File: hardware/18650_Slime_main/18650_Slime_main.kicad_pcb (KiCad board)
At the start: 2 copper layers, 59.8 x 17 mm, 56 parts, among them J1 RJ12, J2 USB_C_Receptacle_USB2.0, J3 Conn_01x04_Male, Q1 2N3904, Q2 CJ2305, Q3 2N3904, Q4 CJ2305, SW1 SW_Push, SW2 SW_Push, SW3 SW_Push, U1 BMI160_Module, U2 ESP32-C3-MINI-1, U3 M3406, U4 SRV05-4, Y1 DNP

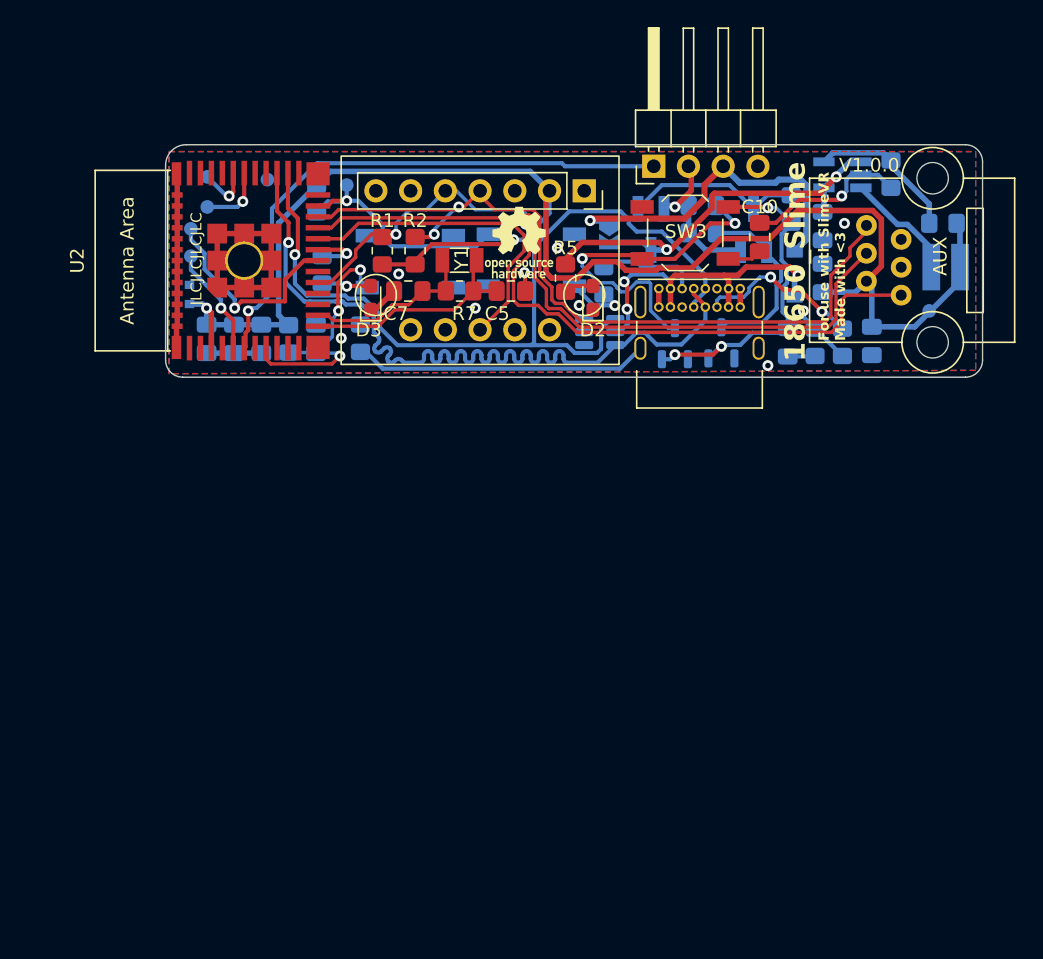
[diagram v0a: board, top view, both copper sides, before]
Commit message: V1.0.0 Release, UNTESTED
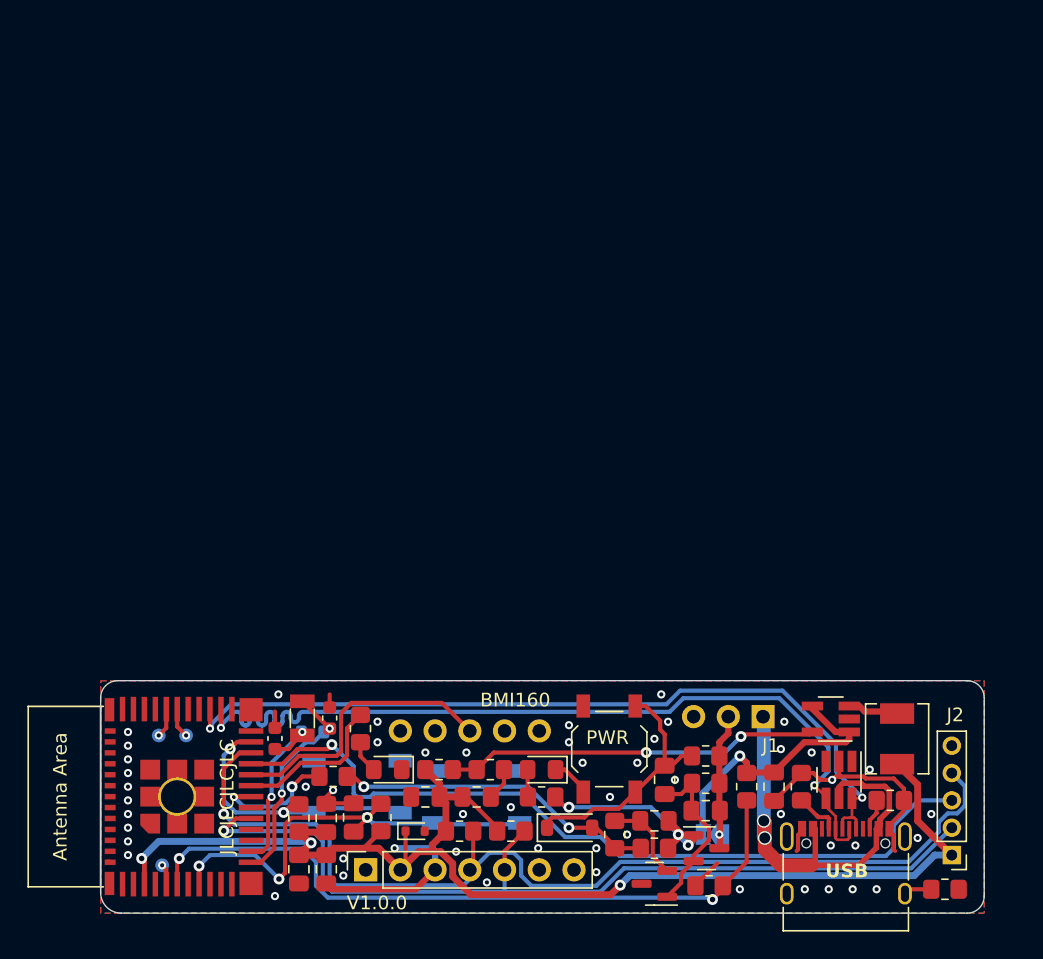
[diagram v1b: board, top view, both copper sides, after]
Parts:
- removed D4: B5819W, Diode_SMD:D_SOD-123
- removed the G*** at (89.6, 62.2)
- removed Q2, Q4: CJ2305, Package_TO_SOT_SMD:SOT-23_Handsoldering
- removed TP3: IO9, TestPoint:TestPoint_Pad_D1.0mm
- removed TP5: IO2, TestPoint:TestPoint_Pad_D1.0mm
- removed TP6: GND, TestPoint:TestPoint_Pad_D1.0mm
- removed TP7: 3v3, TestPoint:TestPoint_Pad_D1.0mm
- added C12: 100nF, Capacitor_SMD:C_0805_2012Metric_Pad1.18x1.45mm_HandSolder, F.Cu at (103.2, 103.8)
- added D5: B5819W, Diode_SMD:D_SOD-123, F.Cu at (93.3, 105.0)
- added G***: LOGO, 18650_Slime:OpenSourceLogo, B.Cu at (69.2, 102.5)
- added R17: 1K, Resistor_SMD:R_0805_2012Metric_Pad1.20x1.40mm_HandSolder, F.Cu at (76.0, 101.2)
- added R18: 120K, Resistor_SMD:R_0805_2012Metric_Pad1.20x1.40mm_HandSolder, F.Cu at (106.2, 102.0)
- added R19: 27K, Resistor_SMD:R_0805_2012Metric_Pad1.20x1.40mm_HandSolder, F.Cu at (103.5, 109.2)
- C1, C2, C3, C4, C8, C9, D1, R10, R11, R12, R14, R3, R4, R6, R8, R9, U3: moved to F.Cu
- C10: value 22uF -> 10uF
- C11: value 10nF -> 1uF; moved to F.Cu
- C5, C7: footprint Capacitor_SMD:C_0805_2012Metric_Pad1.18x1.45mm_HandSolder -> Capacitor_SMD:C_0603_1608Metric
- C6: value 4.7uF -> 10uF; moved to F.Cu
- D2, D3: footprint LED_SMD:LED_0603_1608Metric_Pad1.05x0.95mm_HandSolder -> Diode_SMD:D_0805_2012Metric_Pad1.15x1.40mm_HandSolder
- J1: value RJ12 -> Conn_01x03_Pin; footprint 18650:EVERCOM 5501-660211111 -> Connector_PinHeader_2.54mm:PinHeader_1x03_P2.54mm_Horizontal; moved to B.Cu
- J2: value USB_C_Receptacle_USB2.0 -> Conn_01x05_Pin; footprint Connector_USB:USB_C_Receptacle_GCT_USB4085 -> Connector_PinHeader_2.00mm:PinHeader_1x05_P2.00mm_Vertical
- J3: value Conn_01x04_Male -> USB_C_Receptacle_USB2.0; footprint Connector_PinHeader_2.54mm:PinHeader_1x04_P2.54mm_Horizontal -> Connector_USB:USB_C_Receptacle_XKB_U262-16XN-4BVC11
- L1: footprint Inductor_SMD:L_Wuerth_MAPI-3015 -> 18650:SMMS0420; moved to F.Cu
- Q1: value 2N3904 -> AO3400A; footprint Package_TO_SOT_SMD:SOT-23-3 -> Package_TO_SOT_SMD:SOT-23; moved to F.Cu
- Q3: value 2N3904 -> CJ2305; footprint Package_TO_SOT_SMD:SOT-23-3 -> Package_TO_SOT_SMD:SOT-23; moved to F.Cu
- R1, R2, R5: value 4.7K -> 5.1K
- R13: value 1K -> 10K; moved to F.Cu
- R15: value 100K -> 300K; moved to F.Cu
- R16: value 1M -> 100K; moved to F.Cu
- R7: footprint Resistor_SMD:R_0805_2012Metric_Pad1.20x1.40mm_HandSolder -> Resistor_SMD:R_0603_1608Metric; moved to B.Cu
- U4: footprint Package_TO_SOT_SMD:SOT-23-6 -> Package_TO_SOT_SMD:SOT-23-6_Handsoldering; moved to F.Cu
- moved R4 58.8 mm to (120.8, 109.5), turned to 0 degrees
- moved R8 54.4 mm to (83.8, 100.8), turned to 0 degrees
- moved J3 54.0 mm to (113.5, 108.8), turned to 0 degrees
- moved R9 52.5 mm to (87.5, 100.8), turned to 0 degrees
- moved R16 47.1 mm to (99.5, 106.5)
- moved C8 46.7 mm to (82.8, 102.8), turned to 180 degrees
- moved J2 46.6 mm to (121.2, 107.0), turned to 180 degrees
- moved TP4 46.6 mm to (63.5, 107.8)
- moved C9 45.6 mm to (86.5, 102.8), turned to 0 degrees
- moved R10 45.3 mm to (73.5, 104.3), turned to 90 degrees
- moved JP1 44.7 mm to (103.8, 105.5), turned to 180 degrees
- moved R15 44.5 mm to (96.6, 105.5), turned to -90 degrees
- moved R1 43.5 mm to (89.0, 105.2), turned to 180 degrees
- moved C10 43.4 mm to (99.5, 104.5), turned to 0 degrees
- moved D1 42.6 mm to (82.0, 105.2), turned to 0 degrees
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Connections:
- C10 pad 1: GND -> Net-(Q1-G)
- C10 pad 2: Net-(Q1-C) -> +5V
- C11 pad 1: Net-(Q1-B) -> Net-(Q1-D)
- C11 pad 2: Net-(C11-Pad2) -> Net-(D5-K)
- J1 pad 1: IO8_SCL -> VBUS
- J1 pad 2: GND -> +5P
- J1 pad 3: IO7_INT2 -> GND
- JP1 pad 1: VBUS -> +5P
- Q1 pad 1: GND -> Net-(Q1-D)
- Q1 pad 2: Net-(Q1-B) -> Net-(Q1-G)
- Q1 pad 3: Net-(Q1-C) -> GND
- Q3 pad 1: GND -> +5V
- Q3 pad 2: Net-(Q1-B) -> Net-(Q1-D)
- Q3 pad 3: Net-(Q3-C) -> +5P
- R11 pad 1: Net-(J2-CC2) -> Net-(J3-CC2)
- R12 pad 1: Net-(J2-CC1) -> Net-(J3-CC1)
- R13 pad 1: GND -> Net-(D5-K)
- R13 pad 2: Net-(C11-Pad2) -> +5P
- R14 pad 1: Net-(Q2-G) -> Net-(Q1-D)
- R14 pad 2: Net-(Q1-B) -> +5P
- R15 pad 1: +5P -> Net-(Q1-G)
- R15 pad 2: Net-(Q3-C) -> IO4_ON/OFF
- R16 pad 1: +5P -> IO4_ON/OFF
- R16 pad 2: Net-(Q1-C) -> +5V
- R4 pad 1: Net-(J2-SHIELD) -> Net-(J3-SHIELD)
- SW3 pad 1: Net-(Q1-B) -> GND
- SW3 pad 2: Net-(Q1-C) -> Net-(D5-K)
- TP4 pad 1: UNUSED_IO4 -> UNUSED_IO2
- U2 pad 18: UNUSED_IO4 -> Net-(U2-GPIO4/ADC1_CH4)
- U2 pad 6: B_SENSE -> IO3_B_SENSE
- U4 pad 5: Net-(D4-A) -> VBUS
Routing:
- net IO3_B_SENSE: track 0.00 -> 52.1 mm, vias 0 -> 2
- net B_SENSE: track 40.7 -> 0.00 mm, vias 1 -> 0
- net Net-(Q1-C): track 28.0 -> 0.00 mm, vias 2 -> 0
- net Net-(D4-A): track 25.3 -> 0.00 mm, vias 3 -> 0
- net Net-(Q1-B): track 25.0 -> 0.00 mm, vias 3 -> 0
- net IO4_ON/OFF: track 0.00 -> 23.7 mm, vias 0 -> 2
- net Net-(J2-SHIELD): track 21.2 -> 0.00 mm
- net Net-(D5-K): track 0.00 -> 18.3 mm
- net IO8_SCL: track 57.6 -> 75.5 mm, vias 2 -> 1
- net Net-(U3-FB): track 11.2 -> 27.4 mm, vias 0 -> 2
- net +3V3: track 115.0 -> 99.3 mm, vias 2 -> 3
- net UNUSED_IO4: track 15.6 -> 0.00 mm, vias 1 -> 0
- net GND: track 59.8 -> 45.2 mm, vias 11 -> 53
- net Net-(Q3-C): track 13.7 -> 0.00 mm
- net RESET: track 19.8 -> 32.9 mm
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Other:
- board size 59.8 x 17 mm -> 64.6 x 17 mm
- board text added: "BMI160"
- board text added: "For use with SlimeVR; Made with <3"
- board text added: "GND SCL INT"
- board text added: "IO2"
- board text added: "IO20"
- board text added: "IO21"
- board text added: "PGM"
- board text added: "PWR"
- board text added: "RST"
- board text added: "SDA 3V3"
- board text added: "SW"
- board text added: "USB"
- board text removed: "AUX"
- board text removed: "For use with SlimeVR Made with <3"
